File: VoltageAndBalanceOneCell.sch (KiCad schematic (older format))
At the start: 6 parts, among them Q1 BSS138

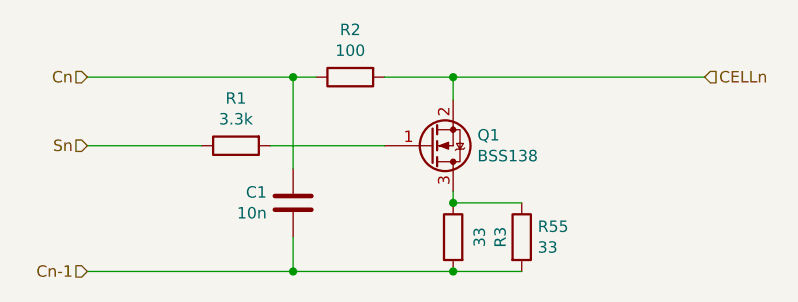
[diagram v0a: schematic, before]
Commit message: petite modif
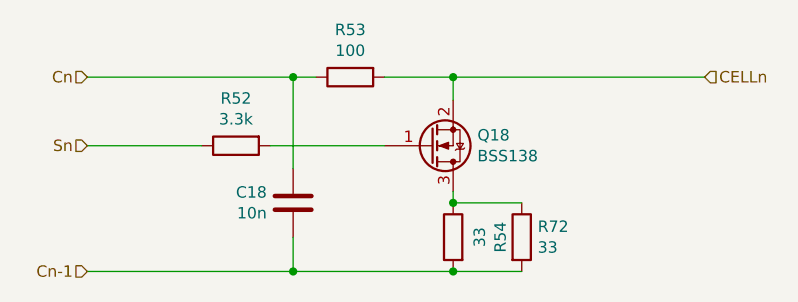
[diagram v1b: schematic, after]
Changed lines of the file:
@@
 AR Path="/5E4D37F6/5E4D5444/5E4D6982" Ref="R50"  Part="1"
 AR Path="/5E4D37F6/5E4D5447/5E4D6982" Ref="R53"  Part="1"
-F 0 "R2" V 3793 1850 50  0000 C CNN
+F 0 "R53" V 3793 1850 50  0000 C CNN
 F 1 "100" V 3884 1850 50  0000 C CNN
 F 2 "Resistor_SMD:R_1206_3216Metric_Pad1.42x1.75mm_HandSolder" V 3930 1850 50  0001 C CNN
@@
 AR Path="/5E4D37F6/5E4D5444/5E4D6989" Ref="R49"  Part="1"
 AR Path="/5E4D37F6/5E4D5447/5E4D6989" Ref="R52"  Part="1"
-F 0 "R1" V 3293 2150 50  0000 C CNN
+F 0 "R52" V 3293 2150 50  0000 C CNN
 F 1 "3.3k" V 3384 2150 50  0000 C CNN
 F 2 "Resistor_SMD:R_1206_3216Metric_Pad1.42x1.75mm_HandSolder" V 3430 2150 39  0001 C CNN
@@
 AR Path="/5E4D37F6/5E4D5444/5E4D6990" Ref="C17"  Part="1"
 AR Path="/5E4D37F6/5E4D5447/5E4D6990" Ref="C18"  Part="1"
-F 0 "C1" H 3865 2446 50  0000 L CNN
+F 0 "C18" H 3865 2446 50  0000 L CNN
 F 1 "10n" H 3865 2355 50  0000 L CNN
 F 2 "Resistor_SMD:R_1206_3216Metric_Pad1.42x1.75mm_HandSolder" H 3788 2250 50  0001 C CNN
@@
 AR Path="/5E4D37F6/5E4D5444/5E4D6997" Ref="Q17"  Part="1"
 AR Path="/5E4D37F6/5E4D5447/5E4D6997" Ref="Q18"  Part="1"
-F 0 "Q1" H 4556 2104 50  0000 L CNN
+F 0 "Q18" H 4556 2104 50  0000 L CNN
 F 1 "BSS138" H 4556 2195 50  0000 L CNN
 F 2 "Package_TO_SOT_SMD:SOT-23" H 4550 2075 50  0001 L CIN
@@
 AR Path="/5E4D37F6/5E4D5444/5E4D699E" Ref="R51"  Part="1"
 AR Path="/5E4D37F6/5E4D5447/5E4D699E" Ref="R54"  Part="1"
-F 0 "R3" V 4243 2550 50  0000 C CNN
+F 0 "R54" V 4243 2550 50  0000 C CNN
 F 1 "33" V 4334 2550 50  0000 C CNN
 F 2 "Resistor_SMD:R_1206_3216Metric_Pad1.42x1.75mm_HandSolder" V 4380 2550 50  0001 C CNN
@@
 AR Path="/5E4D37F6/5E4D5444/5F95DD3D" Ref="R71"  Part="1"
 AR Path="/5E4D37F6/5E4D5447/5F95DD3D" Ref="R72"  Part="1"
-F 0 "R55" H 4820 2596 50  0000 L CNN
+F 0 "R72" H 4820 2596 50  0000 L CNN
 F 1 "33" H 4820 2505 50  0000 L CNN
 F 2 "Resistor_THT:R_Axial_DIN0207_L6.3mm_D2.5mm_P10.16mm_Horizontal" V 4680 2550 50  0001 C CNN

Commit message: tout route sauf voltage channel
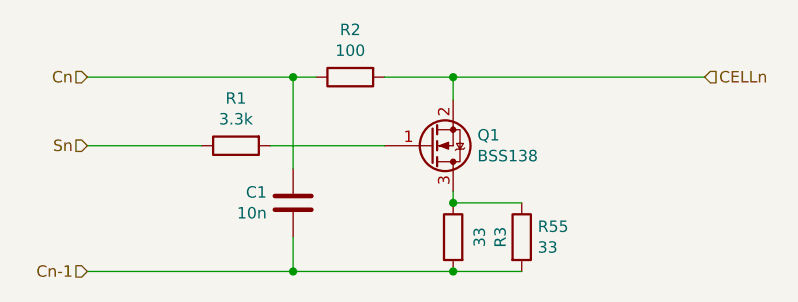
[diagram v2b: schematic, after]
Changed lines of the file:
@@
 AR Path="/5E4D37F6/5E4D5444/5E4D6982" Ref="R50"  Part="1"
 AR Path="/5E4D37F6/5E4D5447/5E4D6982" Ref="R53"  Part="1"
-F 0 "R53" V 3793 1850 50  0000 C CNN
+F 0 "R2" V 3793 1850 50  0000 C CNN
 F 1 "100" V 3884 1850 50  0000 C CNN
 F 2 "Resistor_SMD:R_1206_3216Metric_Pad1.42x1.75mm_HandSolder" V 3930 1850 50  0001 C CNN
@@
 AR Path="/5E4D37F6/5E4D5444/5E4D6989" Ref="R49"  Part="1"
 AR Path="/5E4D37F6/5E4D5447/5E4D6989" Ref="R52"  Part="1"
-F 0 "R52" V 3293 2150 50  0000 C CNN
+F 0 "R1" V 3293 2150 50  0000 C CNN
 F 1 "3.3k" V 3384 2150 50  0000 C CNN
 F 2 "Resistor_SMD:R_1206_3216Metric_Pad1.42x1.75mm_HandSolder" V 3430 2150 39  0001 C CNN
@@
 AR Path="/5E4D37F6/5E4D5444/5E4D6990" Ref="C17"  Part="1"
 AR Path="/5E4D37F6/5E4D5447/5E4D6990" Ref="C18"  Part="1"
-F 0 "C18" H 3865 2446 50  0000 L CNN
+F 0 "C1" H 3865 2446 50  0000 L CNN
 F 1 "10n" H 3865 2355 50  0000 L CNN
 F 2 "Resistor_SMD:R_1206_3216Metric_Pad1.42x1.75mm_HandSolder" H 3788 2250 50  0001 C CNN
@@
 AR Path="/5E4D37F6/5E4D5444/5E4D6997" Ref="Q17"  Part="1"
 AR Path="/5E4D37F6/5E4D5447/5E4D6997" Ref="Q18"  Part="1"
-F 0 "Q18" H 4556 2104 50  0000 L CNN
+F 0 "Q1" H 4556 2104 50  0000 L CNN
 F 1 "BSS138" H 4556 2195 50  0000 L CNN
 F 2 "Package_TO_SOT_SMD:SOT-23" H 4550 2075 50  0001 L CIN
@@
 AR Path="/5E4D37F6/5E4D5444/5E4D699E" Ref="R51"  Part="1"
 AR Path="/5E4D37F6/5E4D5447/5E4D699E" Ref="R54"  Part="1"
-F 0 "R54" V 4243 2550 50  0000 C CNN
+F 0 "R3" V 4243 2550 50  0000 C CNN
 F 1 "33" V 4334 2550 50  0000 C CNN
 F 2 "Resistor_SMD:R_1206_3216Metric_Pad1.42x1.75mm_HandSolder" V 4380 2550 50  0001 C CNN
@@
 AR Path="/5E4D37F6/5E4D5444/5F95DD3D" Ref="R71"  Part="1"
 AR Path="/5E4D37F6/5E4D5447/5F95DD3D" Ref="R72"  Part="1"
-F 0 "R72" H 4820 2596 50  0000 L CNN
+F 0 "R55" H 4820 2596 50  0000 L CNN
 F 1 "33" H 4820 2505 50  0000 L CNN
 F 2 "Resistor_THT:R_Axial_DIN0207_L6.3mm_D2.5mm_P10.16mm_Horizontal" V 4680 2550 50  0001 C CNN
